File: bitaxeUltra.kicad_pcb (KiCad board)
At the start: 4 copper layers, 56.5 x 99.8 mm, 146 parts, among them J1 54-00164, J10 Conn_01x02, J2 Conn_01x02, J3 Conn_01x05, J4 Conn_01x04, J5 TC2030-IDC, J6 Conn_01x04, J7 Conn_01x02, J8 USB_C_Receptacle_USB2.0, J9 Conn_01x04, Q1 CSD17311Q5, Q2 CSD17311Q5, Q4 2N7002K, SW1 GT-TC029B-H025-L1N, SW2 GT-TC029B-H025-L1N, U1 25MHz, U10 DS4432U+, U11 RT9080-33GJ5, U12 ESP32-S3-WROOM-1, U14 BM1366_mode1, U2 TXB0104RGYR, U5 MCP1824T-1802E, U6 MCP1824T-0802E, U7 EMC2101, U8 INA260, U9 TPS40305, Y1 32.768kHz

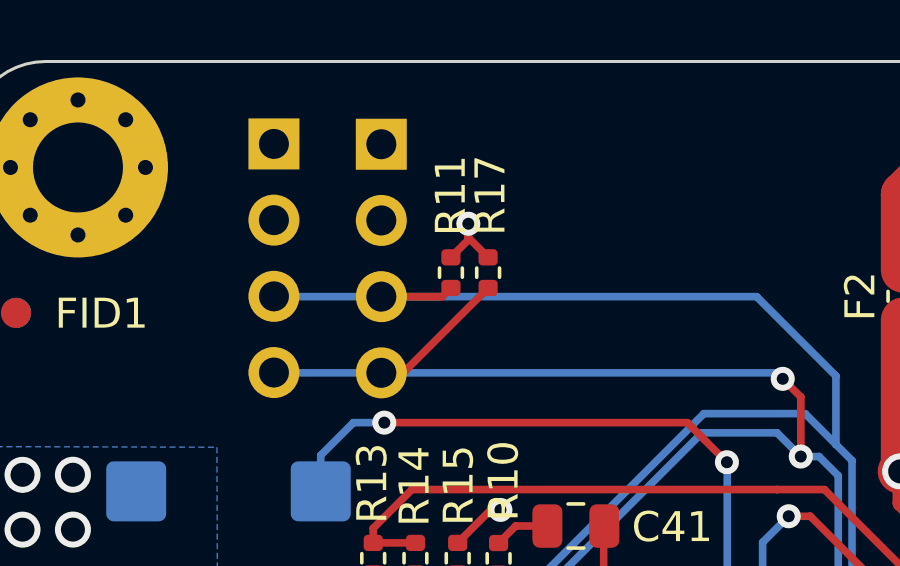
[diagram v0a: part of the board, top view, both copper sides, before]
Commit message: small tweak
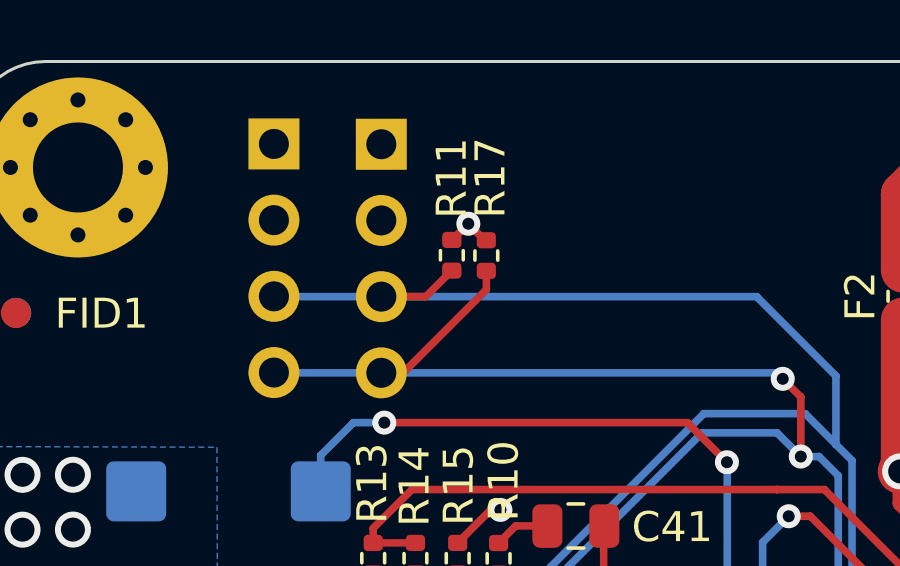
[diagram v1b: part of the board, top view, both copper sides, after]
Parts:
- moved R11 0.58 mm to (93.3, 54.0)
- moved R17 0.57 mm to (94.4, 54.0)
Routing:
- net /3V3: track 78.6 -> 77.4 mm
- net /SDA: track 134.2 -> 134.8 mm
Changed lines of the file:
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@@
 	(footprint "Resistor_SMD:R_0402_1005Metric"
 		(layer "F.Cu")
-		(at 94.48 54.56 90)
+		(at 94.42 53.99 90)
 		(descr "Resistor SMD 0402 (1005 Metric), square (rectangular) end terminal, IPC_7351 nominal, (Body size source: IPC-SM-782 page 72, https://www.pcb-3d.com/wordpress/wp-content/uploads/ipc-sm-782a_amendment_1_and_2.pdf), generated with kicad-footprint-generator")
 		(tags "resistor")
 		(property "Reference" "R17"
-			(at 2.58 0.08 90)
+			(at 2.59 0.14 90)
 			(layer "F.SilkS")
 			(effects
@@
 	(footprint "Resistor_SMD:R_0402_1005Metric"
 		(layer "F.Cu")
-		(at 93.24 54.56 90)
+		(at 93.27 53.98 90)
 		(descr "Resistor SMD 0402 (1005 Metric), square (rectangular) end terminal, IPC_7351 nominal, (Body size source: IPC-SM-782 page 72, https://www.pcb-3d.com/wordpress/wp-content/uploads/ipc-sm-782a_amendment_1_and_2.pdf), generated with kicad-footprint-generator")
 		(tags "resistor")
@@
 	)
 	(segment
-		(start 93.82 53.39)
+		(start 94.37 53.48)
 		(end 93.82 52.93)
 		(width 0.254)
@@
 	)
 	(segment
-		(start 93.24 54.05)
-		(end 93.82 53.47)
-		(width 0.254)
-		(layer "F.Cu")
-		(net 8)
-	)
-	(segment
 		(start 115.493 61.343)
 		(end 115.08 60.93)
@@
 	)
 	(segment
-		(start 93.82 53.47)
-		(end 93.82 52.93)
-		(width 0.254)
-		(layer "F.Cu")
-		(net 8)
-	)
-	(segment
 		(start 95.19 98.565)
 		(end 95.19 97.56)
@@
 	)
 	(segment
+		(start 94.42 53.48)
+		(end 94.37 53.48)
+		(width 0.254)
+		(layer "F.Cu")
+		(net 8)
+	)
+	(segment
 		(start 113.94095 62.4402)
 		(end 115.4928 62.4402)
@@
 	)
 	(segment
-		(start 82.99 84.925)
-		(end 84.52 83.395)
-		(width 0.508)
+		(start 93.28 53.47)
+		(end 93.82 52.93)
+		(width 0.254)
 		(layer "F.Cu")
 		(net 8)
 	)
 	(segment
-		(start 94.48 54.05)
-		(end 93.82 53.39)
-		(width 0.254)
+		(start 82.99 84.925)
+		(end 84.52 83.395)
+		(width 0.508)
 		(layer "F.Cu")
 		(net 8)
@@
 	)
 	(segment
+		(start 93.27 53.47)
+		(end 93.28 53.47)
+		(width 0.254)
+		(layer "F.Cu")
+		(net 8)
+	)
+	(segment
 		(start 131.05 85.7)
 		(end 131.05 84.56)
@@
 	)
 	(segment
-		(start 93.79 52.9)
-		(end 91 52.9)
+		(start 93.82 52.93)
+		(end 93.85 52.9)
 		(width 1.5)
 		(layer "In2.Cu")
@@
 	)
 	(segment
-		(start 90.92 52.82)
-		(end 87.35 52.82)
+		(start 93.79 52.9)
+		(end 91 52.9)
 		(width 1.5)
 		(layer "In2.Cu")
@@
 	)
 	(segment
-		(start 93.85 52.9)
-		(end 93.82 52.93)
+		(start 109.13 52.9)
+		(end 111.16 54.93)
 		(width 1.5)
 		(layer "In2.Cu")
@@
 	)
 	(segment
-		(start 91 52.9)
-		(end 90.92 52.82)
+		(start 90.92 52.82)
+		(end 87.35 52.82)
 		(width 1.5)
 		(layer "In2.Cu")
@@
 	)
 	(segment
-		(start 93.82 52.93)
-		(end 93.79 52.9)
+		(start 91 52.9)
+		(end 90.92 52.82)
 		(width 1.5)
 		(layer "In2.Cu")
@@
 	)
 	(segment
-		(start 109.13 52.9)
-		(end 93.85 52.9)
+		(start 93.85 52.9)
+		(end 109.13 52.9)
 		(width 1.5)
 		(layer "In2.Cu")
@@
 	)
 	(segment
-		(start 111.16 54.93)
-		(end 109.13 52.9)
+		(start 93.82 52.93)
+		(end 93.79 52.9)
 		(width 1.5)
 		(layer "In2.Cu")
@@
 	)
 	(segment
-		(start 101.36 120.659)
-		(end 102.3718 119.6472)
+		(start 93.27 54.49)
+		(end 92.4 55.36)
 		(width 0.254)
 		(layer "F.Cu")
@@
 	)
 	(segment
-		(start 89.58 98.5638)
-		(end 90.2312 99.215)
+		(start 101.36 120.659)
+		(end 102.3718 119.6472)
 		(width 0.254)
 		(layer "F.Cu")
@@
 	)
 	(segment
-		(start 93.24 55.07)
-		(end 92.95 55.36)
+		(start 89.58 98.5638)
+		(end 90.2312 99.215)
 		(width 0.254)
 		(layer "F.Cu")
@@
 	)
 	(segment
-		(start 92.95 55.36)
+		(start 92.4 55.36)
 		(end 90.92 55.36)
 		(width 0.254)
@@
 	)
 	(segment
+		(start 94.42 55.13)
+		(end 91.65 57.9)
+		(width 0.254)
+		(layer "F.Cu")
+		(net 64)
+	)
+	(segment
 		(start 89.85 96.26)
 		(end 90.89 97.3)
@@
 	)
 	(segment
-		(start 94.48 55.07)
-		(end 91.65 57.9)
+		(start 91.65 57.9)
+		(end 90.92 57.9)
 		(width 0.254)
 		(layer "F.Cu")
@@
 	)
 	(segment
+		(start 94.42 54.5)
+		(end 94.42 55.13)
+		(width 0.254)
+		(layer "F.Cu")
+		(net 64)
+	)
+	(segment
 		(start 101.186 119.888)
 		(end 101.7218 119.3522)
@@
 		(width 0.254)
 		(layer "F.Cu")
-		(net 64)
-	)
-	(segment
-		(start 91.65 57.9)
-		(end 90.92 57.9)
-		(width 0.254)
-		(layer "F.Cu")
